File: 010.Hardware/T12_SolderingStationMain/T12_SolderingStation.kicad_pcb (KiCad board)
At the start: 2 copper layers, 80 x 23 mm, 51 parts, among them J1 USB_C_Receptacle_USB2.0, J2 AVR-ISP-6, J3 Conn_01x04_Male, J4 Conn_01x05_Female, SW1 SW_DPST_Temperature, SW2 RotaryEncoder_2, U1 MP1584EN, U2 CH224D, U3 ATmega328P-A, U4 OPA2333xxD, Y1 16mHz

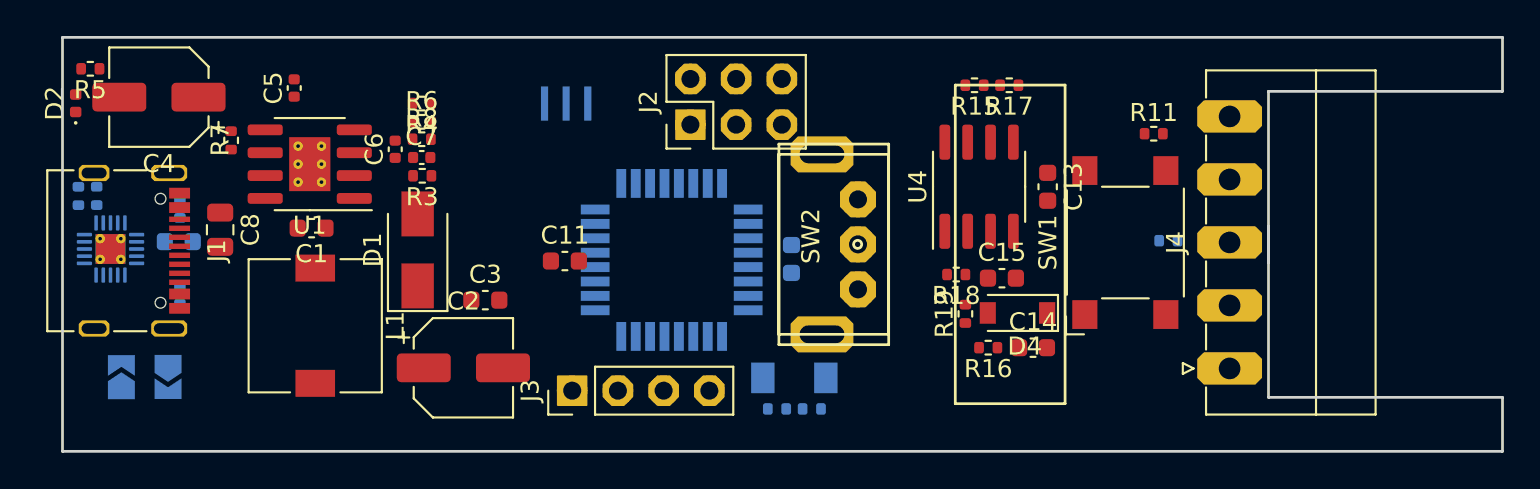
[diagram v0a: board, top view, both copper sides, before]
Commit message: 完善图纸
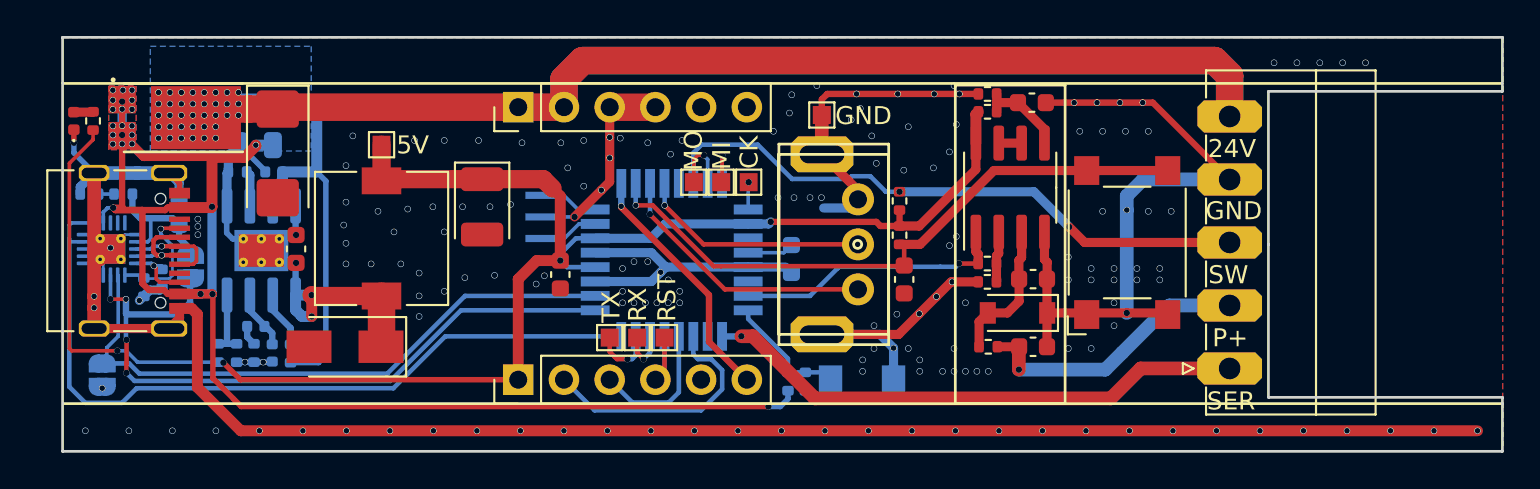
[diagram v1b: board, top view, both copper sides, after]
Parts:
- removed J2: AVR-ISP-6, Connector_PinHeader_2.54mm:PinHeader_2x03_P2.54mm_Vertical
- removed J3: Conn_01x04_Male, Connector_PinHeader_2.54mm:PinHeader_1x04_P2.54mm_Vertical
- added D5: SDT10A45P5, My_Library:PowerDI5, F.Cu at (86.4, 80.3)
- added J5: Conn_01x06_Female, Connector_PinHeader_2.54mm:PinHeader_1x06_P2.54mm_Vertical, F.Cu at (106.8, 94.9)
- added J6: Conn_01x06_Female, Connector_PinHeader_2.54mm:PinHeader_1x06_P2.54mm_Vertical, F.Cu at (106.8, 79.8)
- added TP1: VCC, TestPoint:TestPoint_Pad_1.0x1.0mm, F.Cu at (99.2, 81.8)
- added TP2: MISO, TestPoint:TestPoint_Pad_1.0x1.0mm, F.Cu at (118.1, 83.9)
- added TP3: MOSI, TestPoint:TestPoint_Pad_1.0x1.0mm, F.Cu at (116.6, 83.9)
- added TP4: SCK, TestPoint:TestPoint_Pad_1.0x1.0mm, F.Cu at (119.6, 83.9)
- added TP5: RST, TestPoint:TestPoint_Pad_1.0x1.0mm, F.Cu at (115.0, 92.6)
- added TP6: GND, TestPoint:TestPoint_Pad_1.0x1.0mm, F.Cu at (123.7, 80.2)
- added TP7: TXD, TestPoint:TestPoint_Pad_1.0x1.0mm, F.Cu at (111.9, 92.6)
- added TP8: RXD, TestPoint:TestPoint_Pad_1.0x1.0mm, F.Cu at (113.4, 92.6)
- C2: footprint Capacitor_SMD:CP_Elec_5x5.7 -> Capacitor_Tantalum_SMD:CP_EIA-3528-21_Kemet-B
- C4: footprint Capacitor_SMD:CP_Elec_5x5.7 -> Capacitor_Tantalum_SMD:CP_EIA-6032-28_Kemet-C
- C5, C6, C7, C8, R3, R4, R6, R7, R8, U1: moved to B.Cu
- JP1, JP2: footprint Jumper:SolderJumper-2_P1.3mm_Open_TrianglePad1.0x1.5mm -> Jumper:SolderJumper-2_P1.3mm_Open_RoundedPad1.0x1.5mm
- R14: moved to F.Cu
- moved C11 18.9 mm to (128.3, 89.3), turned to -90 degrees
- moved R4 17.9 mm to (90.2, 93.4), turned to 90 degrees
- moved R6 16.5 mm to (91.2, 93.4), turned to -90 degrees
- moved R11 15.2 mm to (128.0, 86.9), turned to -90 degrees
- moved R14 15.1 mm to (128.0, 85.0), turned to 90 degrees
- moved R8 15.1 mm to (92.2, 93.4), turned to -90 degrees
- moved C7 13.7 mm to (93.2, 93.4), turned to -90 degrees
- moved C6 12.5 mm to (92.3, 91.9), turned to 180 degrees
- moved R3 12.3 mm to (94.2, 93.4), turned to 90 degrees
- moved C2 9.00 mm to (104.8, 85.3), turned to -90 degrees
- moved C4 7.31 mm to (93.5, 82.3), turned to -90 degrees
- moved D1 6.73 mm to (97.2, 93.1), turned to 180 degrees
- moved Y1 6.43 mm to (108.2, 85.9), turned to -90 degrees
- moved JP1 6.25 mm to (88.6, 88.6), turned to 90 degrees
- moved L1 6.09 mm to (99.2, 87.0), turned to 90 degrees
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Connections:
- C4 pad 1: VBUS -> +24V
- C5 pad 1: VBUS -> +24V
- J4 pad 1: VBUS -> /ADC2
- J4 pad 4: /ADC2 -> GND
- J4 pad 5: GND -> +24V
- R3 pad 1: VBUS -> +24V
- SW2 pad B: /D6 -> /D8
- U1 pad 7: VBUS -> +24V
- U3 pad 12: /D6 -> /D8
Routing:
- net GND: track 0.00 -> 217.8 mm, vias 0 -> 167
- net +24V: track 0.00 -> 145.4 mm, vias 0 -> 36
- net VCC: track 0.00 -> 94.5 mm, vias 0 -> 4
- net VBUS: track 0.00 -> 92.6 mm, vias 0 -> 24
- net /CFG1: track 0.00 -> 46.6 mm
- net /CFG2: track 0.00 -> 39.4 mm, vias 0 -> 4
- net /D6: track 0.00 -> 35.4 mm, vias 0 -> 1
- net /CFG3: track 0.00 -> 34.5 mm
- net /D10: track 0.00 -> 34.1 mm, vias 0 -> 3
- net /ADC2: track 0.00 -> 30.3 mm, vias 0 -> 1
- net P+: track 0.00 -> 15.7 mm, vias 0 -> 1
- net /ADC0: track 0.00 -> 15.5 mm, vias 0 -> 1
- net /D7: track 0.00 -> 15.0 mm, vias 0 -> 1
- net /SDA: track 0.00 -> 14.7 mm
- net /BEEP: track 0.00 -> 13.8 mm, vias 0 -> 1
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- added copper zone on B.Cu, net +24V
- added copper zone on B.Cu, net GND
- added copper zone on F.Cu, net GND
- added copper zone on B.Cu, net VBUS
- added copper zone on F.Cu, net VBUS
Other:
- outline, holes or cut-outs redrawn
- board text added: "24V"
- board text added: "5V"
- board text added: "CK"
- board text added: "GND"
- board text added: "MI"
- board text added: "MO"
- board text added: "P+"
- board text added: "RST"
- board text added: "RX"
- board text added: "SER"
- board text added: "SW"
- board text added: "TX"
